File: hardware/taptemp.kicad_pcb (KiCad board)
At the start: 2 copper layers, 80 x 50 mm, 21 parts, among them J1 Conn_01x04_Pin, J2 Conn_01x02, SW1 SW_Push, SW2 SW_Push, SW3 SW_Push, SW4 SW_Push, U1 MCCOG21605D6W-BNMLWI, U2 STM8L152C6T6TR, Y1 Crystal

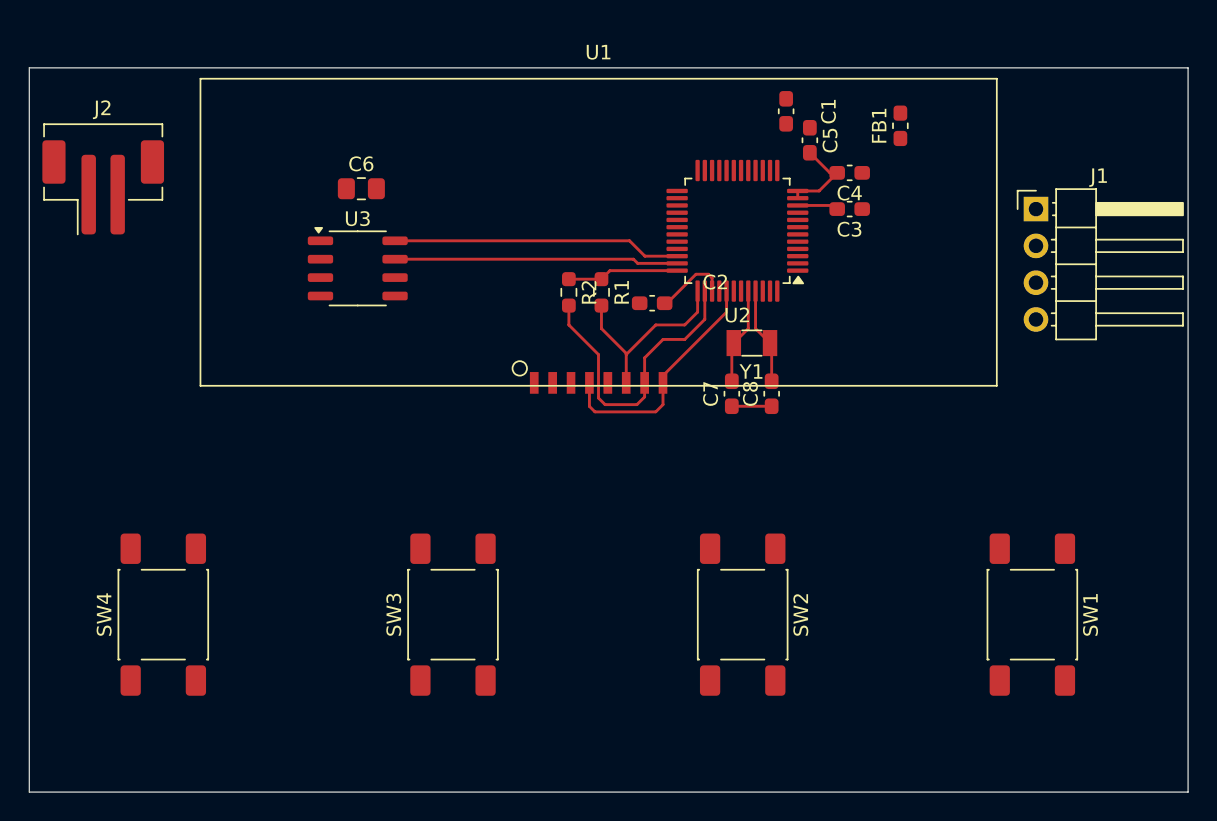
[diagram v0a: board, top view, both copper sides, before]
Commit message: dev: completed routing
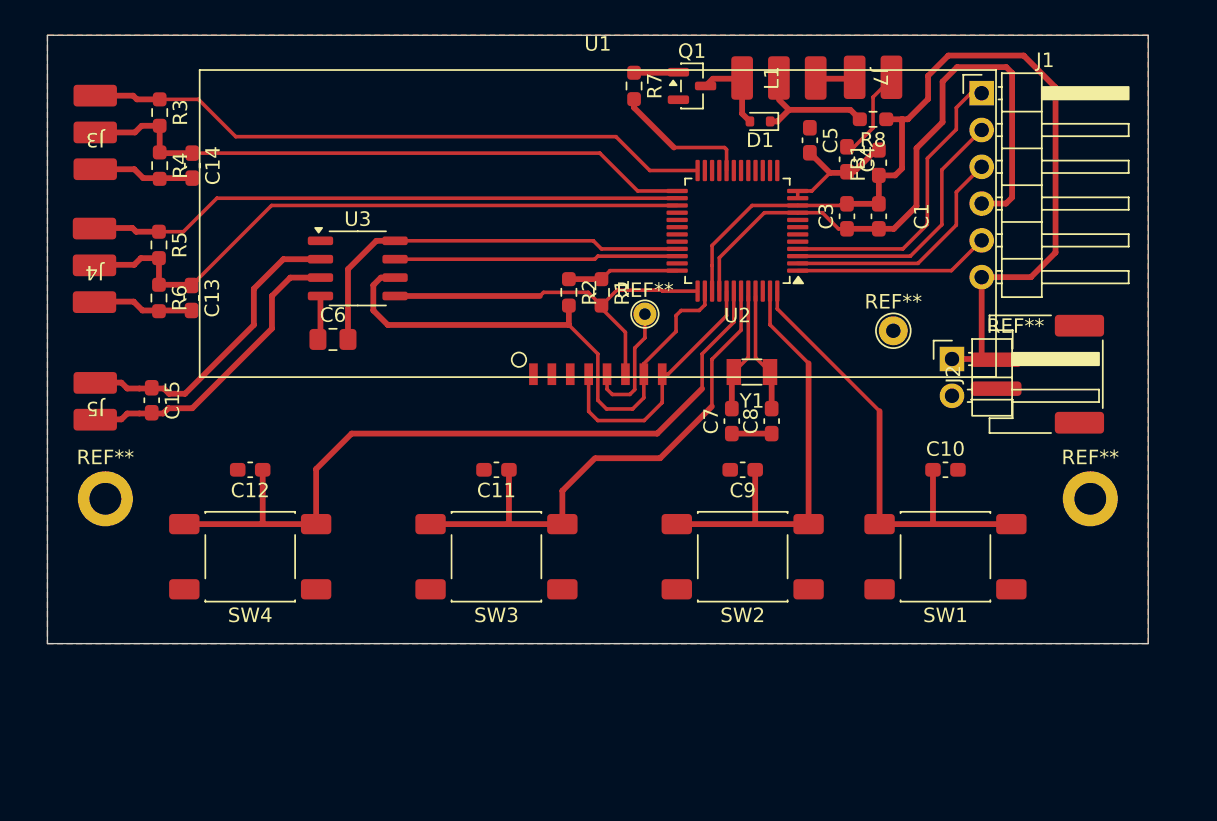
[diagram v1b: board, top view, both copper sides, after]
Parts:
- removed C2: 100n, Capacitor_SMD:C_0603_1608Metric_Pad1.08x0.95mm_HandSolder
- added C10: 100n, Capacitor_SMD:C_0603_1608Metric_Pad1.08x0.95mm_HandSolder, F.Cu at (176.0, 100.0)
- added C11: 100n, Capacitor_SMD:C_0603_1608Metric_Pad1.08x0.95mm_HandSolder, F.Cu at (145.0, 100.0)
- added C12: 100n, Capacitor_SMD:C_0603_1608Metric_Pad1.08x0.95mm_HandSolder, F.Cu at (128.0, 100.0)
- added C13: 1n, Capacitor_SMD:C_0603_1608Metric_Pad1.08x0.95mm_HandSolder, F.Cu at (124.0, 88.1)
- added C14: 1n, Capacitor_SMD:C_0603_1608Metric_Pad1.08x0.95mm_HandSolder, F.Cu at (124.0, 79.0)
- added C15: NM, Capacitor_SMD:C_0603_1608Metric_Pad1.08x0.95mm_HandSolder, F.Cu at (121.2, 95.2)
- added C9: 100n, Capacitor_SMD:C_0603_1608Metric_Pad1.08x0.95mm_HandSolder, F.Cu at (162.0, 100.0)
- added D1: 1N4148WT, Diode_SMD:D_SOD-523, F.Cu at (163.2, 76.0)
- added J3: Pad_1x03, TapTemp:Pad1x03, F.Cu at (117.3, 76.7)
- added J4: Pad_1x03, TapTemp:Pad1x03, F.Cu at (117.2, 85.9)
- added J5: Pad_1x02, TapTemp:Pad1x02, F.Cu at (117.3, 95.3)
- added J7: Conn_01x02, TapTemp:Pad1x02, F.Cu at (171.0, 72.9)
- added L1: ~, TapTemp:Pad1x03, F.Cu at (164.5, 73.0)
- added Q1: BC847, Package_TO_SOT_SMD:SOT-23, F.Cu at (158.5, 73.5)
- added R3: NM, Resistor_SMD:R_0603_1608Metric_Pad0.98x0.95mm_HandSolder, F.Cu at (121.8, 75.3)
- added R4: 4700, Resistor_SMD:R_0603_1608Metric_Pad0.98x0.95mm_HandSolder, F.Cu at (121.8, 79.0)
- added R5: NM, Resistor_SMD:R_0603_1608Metric_Pad0.98x0.95mm_HandSolder, F.Cu at (121.7, 84.5)
- added R6: 4700, Resistor_SMD:R_0603_1608Metric_Pad0.98x0.95mm_HandSolder, F.Cu at (121.7, 88.1)
- added R7: 10k, Resistor_SMD:R_0603_1608Metric_Pad0.98x0.95mm_HandSolder, F.Cu at (154.5, 73.5)
- added R8: 2, Resistor_SMD:R_0603_1608Metric_Pad0.98x0.95mm_HandSolder, F.Cu at (171.0, 75.8)
- added REF**: PinHeader_1x02_P2.54mm_Horizontal, Connector_PinHeader_2.54mm:PinHeader_1x02_P2.54mm_Horizontal, F.Cu at (176.4, 92.3)
- added REF**: MountingHole_2.2mm_M2_DIN965_Pad, MountingHole:MountingHole_2.2mm_M2_DIN965_Pad, F.Cu at (118.0, 102.0)
- added REF**: TestPoint_THTPad_D1.5mm_Drill0.7mm, TestPoint:TestPoint_THTPad_D1.5mm_Drill0.7mm, F.Cu at (155.2, 89.2)
- added REF**: MountingHole_2.2mm_M2_DIN965_Pad, MountingHole:MountingHole_2.2mm_M2_DIN965_Pad, F.Cu at (186.0, 102.0)
- added REF**: TestPoint_THTPad_D2.0mm_Drill1.0mm, TestPoint:TestPoint_THTPad_D2.0mm_Drill1.0mm, F.Cu at (172.4, 90.4)
- C6: value 100nF -> 100n
- J1: value Conn_01x04_Pin -> HDR 1x06; footprint Connector_PinHeader_2.54mm:PinHeader_1x04_P2.54mm_Horizontal -> Connector_PinHeader_2.54mm:PinHeader_1x06_P2.54mm_Horizontal
- J2: footprint Connector_JST:JST_PH_B2B-PH-SM4-TB_1x02-1MP_P2.00mm_Vertical -> Connector_JST:JST_PH_S2B-PH-SM4-TB_1x02-1MP_P2.00mm_Horizontal
- U1: footprint MIDAS:MCCOG21605D6W -> TapTemp:MCCOG21605D6W
- moved J2 65.8 mm to (182.3, 93.4), turned to 90 degrees
- moved SW2 20.4 mm to (162.0, 106.0), turned to 180 degrees
- moved SW3 17.5 mm to (145.0, 106.0), turned to 180 degrees
- moved C6 10.6 mm to (133.7, 91.0)
- moved C1 9.67 mm to (171.4, 82.5)
- moved J1 8.84 mm to (178.5, 74.0)
- moved SW1 7.21 mm to (176.0, 106.0), turned to 180 degrees
- moved SW4 7.21 mm to (128.0, 106.0), turned to 180 degrees
- moved FB1 2.95 mm to (171.4, 78.8)
- moved Y1 2.00 mm to (162.6, 93.2)
- moved C7 1.89 mm to (161.2, 96.6)
- moved C8 1.89 mm to (164.0, 96.6)
- moved C4 0.96 mm to (169.2, 78.6), turned to -90 degrees
- moved U1 0.60 mm to (152.0, 83.0)
- moved C3 0.53 mm to (169.2, 82.5), turned to 90 degrees
- renumbered SW3 to SW2, SW2 to SW3
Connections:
- C6 pad 2: Net-(U2A-PD5) -> Net-(U2A-PD4)
- J1 pad 1: /NRST -> /DRX
- J1 pad 2: GND -> /DTX
- J1 pad 3: /SWIM -> /NRST
- J1 pad 4: VDD -> GND
- SW3 pad 2: unconnected-(SW2-Pad2) -> Net-(U2A-PC4)
- SW4 pad 2: unconnected-(SW4-Pad2) -> Net-(U2A-PC3)
- U2 pad 20: unconnected-(U2A-PD0-Pad20) -> Net-(U2A-PD0)
- U2 pad 24: unconnected-(U2A-PB0-Pad24) -> Net-(J3-Pin_3)
- U2 pad 25: unconnected-(U2A-PB1-Pad25) -> Net-(J3-Pin_2)
- U2 pad 26: unconnected-(U2A-PB2-Pad26) -> Net-(J4-Pin_3)
- U2 pad 27: unconnected-(U2A-PB3-Pad27) -> Net-(J4-Pin_2)
- U2 pad 3: unconnected-(U2A-PA2/OSC_IN-Pad3) -> /DTX
- U2 pad 33: unconnected-(U2A-PD4-Pad33) -> Net-(U2A-PD4)
- U2 pad 35: Net-(U2A-PD6) -> unconnected-(U2A-PD6-Pad35)
- U2 pad 4: unconnected-(U2A-PA3/OSC_OUT-Pad4) -> /DRX
- U2 pad 42: unconnected-(U2A-PC3-Pad42) -> Net-(U2A-PC3)
- U2 pad 43: unconnected-(U2A-PC4-Pad43) -> Net-(U2A-PC4)
- U3 pad 2: unconnected-(U3-AC0-Pad2) -> Net-(J5-Pin_2)
- U3 pad 3: unconnected-(U3-AC1-Pad3) -> Net-(J5-Pin_1)
- U3 pad 7: Net-(U2A-PD6) -> Net-(U2A-PD5)
- U3 pad 8: Net-(U2A-PD5) -> Net-(U2A-PD4)
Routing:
- net GND: track 2.75 -> 77.3 mm
- net VDD: track 7.63 -> 64.2 mm
- net Net-(U2A-PC3): track 0.00 -> 53.3 mm
- net Net-(J4-Pin_2): track 0.00 -> 43.9 mm
- net Net-(J3-Pin_3): track 0.00 -> 43.4 mm
- net Net-(J3-Pin_2): track 0.00 -> 42.7 mm
- net Net-(J4-Pin_3): track 0.00 -> 40.9 mm
- net Net-(U2A-PC4): track 0.00 -> 36.7 mm
- net Net-(U2A-PE7): track 0.00 -> 31.9 mm
- net Net-(U2A-PE6): track 0.00 -> 30.1 mm
- net Net-(U2A-PD4): track 0.00 -> 29.1 mm
- net /DRX: track 0.00 -> 20.7 mm
- net Net-(J5-Pin_2): track 0.00 -> 20.5 mm
- net Net-(J5-Pin_1): track 0.00 -> 20.2 mm
- net Net-(U2A-PD6): track 19.6 -> 0.00 mm
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- added copper zone on B.Cu, net GND
- added copper zone on F.Cu, net GND
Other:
- board size 80 x 50 mm -> 76 x 42 mm
